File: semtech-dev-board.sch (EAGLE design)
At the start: 58 parts, among them Q1 BSS123, U1 SEMTECH_SX1236, U3 MIC5219 3.3V, X1 BU-SMA-G, X2 BU-SMA-G, X3 BU-SMA-G, X4 BU-SMA-G

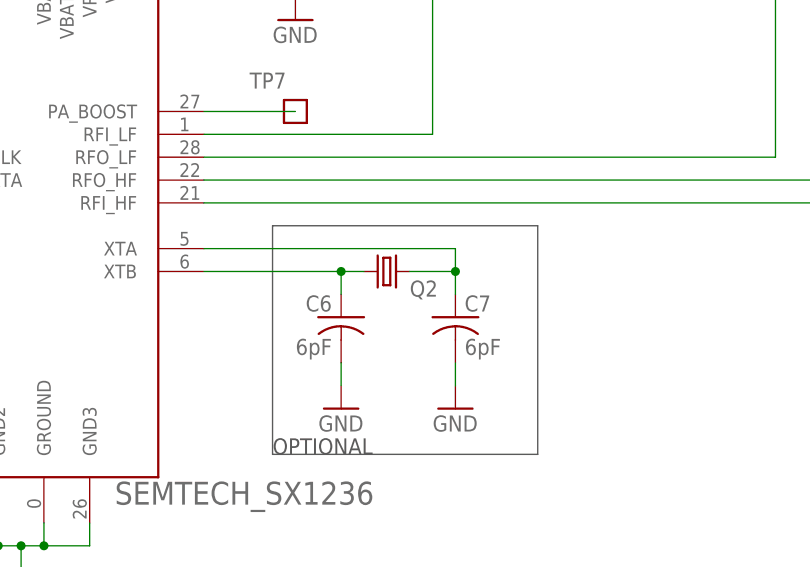
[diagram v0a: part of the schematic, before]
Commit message: minor edits
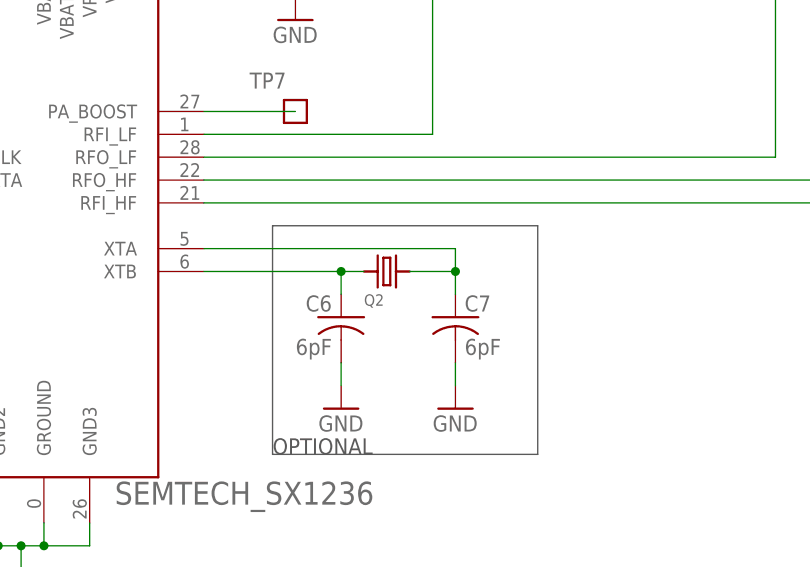
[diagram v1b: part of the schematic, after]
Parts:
- Q2: device crystal:CRYSTALSM49 -> low-gain-radio:CRYSTAL2.5X2.0MM
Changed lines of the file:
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@@
 <grid distance="0.1" unitdist="inch" unit="inch" style="lines" multiple="1" display="no" altdistance="0.01" altunitdist="inch" altunit="inch"/>
 <layers>
-<layer number="1" name="Top" color="4" fill="1" visible="no" active="no"/>
-<layer number="2" name="Route2" color="1" fill="3" visible="no" active="no"/>
-<layer number="3" name="Route3" color="4" fill="3" visible="no" active="no"/>
-<layer number="4" name="Route4" color="1" fill="4" visible="no" active="no"/>
-<layer number="5" name="Route5" color="4" fill="4" visible="no" active="no"/>
-<layer number="6" name="Route6" color="1" fill="8" visible="no" active="no"/>
-<layer number="7" name="Route7" color="4" fill="8" visible="no" active="no"/>
-<layer number="8" name="Route8" color="1" fill="2" visible="no" active="no"/>
-<layer number="9" name="Route9" color="4" fill="2" visible="no" active="no"/>
-<layer number="10" name="Route10" color="1" fill="7" visible="no" active="no"/>
-<layer number="11" name="Route11" color="4" fill="7" visible="no" active="no"/>
-<layer number="12" name="Route12" color="1" fill="5" visible="no" active="no"/>
-<layer number="13" name="Route13" color="4" fill="5" visible="no" active="no"/>
-<layer number="14" name="Route14" color="1" fill="6" visible="no" active="no"/>
-<layer number="15" name="Route15" color="4" fill="6" visible="no" active="no"/>
-<layer number="16" name="Bottom" color="1" fill="1" visible="no" active="no"/>
-<layer number="17" name="Pads" color="2" fill="1" visible="no" active="no"/>
-<layer number="18" name="Vias" color="2" fill="1" visible="no" active="no"/>
-<layer number="19" name="Unrouted" color="6" fill="1" visible="no" active="no"/>
-<layer number="20" name="Dimension" color="15" fill="1" visible="no" active="no"/>
-<layer number="21" name="tPlace" color="7" fill="1" visible="no" active="no"/>
-<layer number="22" name="bPlace" color="7" fill="1" visible="no" active="no"/>
-<layer number="23" name="tOrigins" color="15" fill="1" visible="no" active="no"/>
-<layer number="24" name="bOrigins" color="15" fill="1" visible="no" active="no"/>
-<layer number="25" name="tNames" color="7" fill="1" visible="no" active="no"/>
-<layer number="26" name="bNames" color="7" fill="1" visible="no" active="no"/>
-<layer number="27" name="tValues" color="7" fill="1" visible="no" active="no"/>
-<layer number="28" name="bValues" color="7" fill="1" visible="no" active="no"/>
+<layer number="1" name="Top" color="4" fill="1" visible="yes" active="no"/>
+<layer number="2" name="Route2" color="1" fill="3" visible="yes" active="no"/>
+<layer number="3" name="Route3" color="4" fill="3" visible="yes" active="no"/>
+<layer number="4" name="Route4" color="1" fill="4" visible="yes" active="no"/>
+<layer number="5" name="Route5" color="4" fill="4" visible="yes" active="no"/>
+<layer number="6" name="Route6" color="1" fill="8" visible="yes" active="no"/>
+<layer number="7" name="Route7" color="4" fill="8" visible="yes" active="no"/>
+<layer number="8" name="Route8" color="1" fill="2" visible="yes" active="no"/>
+<layer number="9" name="Route9" color="4" fill="2" visible="yes" active="no"/>
+<layer number="10" name="Route10" color="1" fill="7" visible="yes" active="no"/>
+<layer number="11" name="Route11" color="4" fill="7" visible="yes" active="no"/>
+<layer number="12" name="Route12" color="1" fill="5" visible="yes" active="no"/>
+<layer number="13" name="Route13" color="4" fill="5" visible="yes" active="no"/>
+<layer number="14" name="Route14" color="1" fill="6" visible="yes" active="no"/>
+<layer number="15" name="Route15" color="4" fill="6" visible="yes" active="no"/>
+<layer number="16" name="Bottom" color="1" fill="1" visible="yes" active="no"/>
+<layer number="17" name="Pads" color="2" fill="1" visible="yes" active="no"/>
+<layer number="18" name="Vias" color="2" fill="1" visible="yes" active="no"/>
+<layer number="19" name="Unrouted" color="6" fill="1" visible="yes" active="no"/>
+<layer number="20" name="Dimension" color="15" fill="1" visible="yes" active="no"/>
+<layer number="21" name="tPlace" color="7" fill="1" visible="yes" active="no"/>
+<layer number="22" name="bPlace" color="7" fill="1" visible="yes" active="no"/>
+<layer number="23" name="tOrigins" color="15" fill="1" visible="yes" active="no"/>
+<layer number="24" name="bOrigins" color="15" fill="1" visible="yes" active="no"/>
+<layer number="25" name="tNames" color="7" fill="1" visible="yes" active="no"/>
+<layer number="26" name="bNames" color="7" fill="1" visible="yes" active="no"/>
+<layer number="27" name="tValues" color="7" fill="1" visible="yes" active="no"/>
+<layer number="28" name="bValues" color="7" fill="1" visible="yes" active="no"/>
 <layer number="29" name="tStop" color="7" fill="3" visible="no" active="no"/>
 <layer number="30" name="bStop" color="7" fill="6" visible="no" active="no"/>
@@
 <layer number="35" name="tGlue" color="7" fill="4" visible="no" active="no"/>
 <layer number="36" name="bGlue" color="7" fill="5" visible="no" active="no"/>
-<layer number="37" name="tTest" color="7" fill="1" visible="no" active="no"/>
-<layer number="38" name="bTest" color="7" fill="1" visible="no" active="no"/>
+<layer number="37" name="tTest" color="7" fill="1" visible="yes" active="no"/>
+<layer number="38" name="bTest" color="7" fill="1" visible="yes" active="no"/>
 <layer number="39" name="tKeepout" color="4" fill="11" visible="no" active="no"/>
 <layer number="40" name="bKeepout" color="1" fill="11" visible="no" active="no"/>
@@
 <layer number="44" name="Drills" color="7" fill="1" visible="no" active="no"/>
 <layer number="45" name="Holes" color="7" fill="1" visible="no" active="no"/>
-<layer number="46" name="Milling" color="3" fill="1" visible="no" active="no"/>
-<layer number="47" name="Measures" color="7" fill="1" visible="no" active="no"/>
-<layer number="48" name="Document" color="7" fill="1" visible="no" active="no"/>
-<layer number="49" name="Reference" color="7" fill="1" visible="no" active="no"/>
-<layer number="50" name="dxf" color="7" fill="1" visible="no" active="no"/>
-<layer number="51" name="tDocu" color="7" fill="1" visible="no" active="no"/>
-<layer number="52" name="bDocu" color="7" fill="1" visible="no" active="no"/>
-<layer number="53" name="tGND_GNDA" color="7" fill="1" visible="no" active="no"/>
-<layer number="54" name="bGND_GNDA" color="7" fill="1" visible="no" active="no"/>
-<layer number="56" name="wert" color="7" fill="1" visible="no" active="no"/>
-<layer number="57" name="tCAD" color="7" fill="1" visible="no" active="no"/>
-<layer number="58" name="b3D" color="7" fill="1" visible="no" active="no"/>
-<layer number="59" name="Invisible" color="7" fill="1" visible="no" active="no"/>
-<layer number="60" name="bCarbon" color="7" fill="1" visible="no" active="no"/>
-<layer number="61" name="stand" color="7" fill="1" visible="no" active="no"/>
+<layer number="46" name="Milling" color="3" fill="1" visible="yes" active="no"/>
+<layer number="47" name="Measures" color="7" fill="1" visible="yes" active="no"/>
+<layer number="48" name="Document" color="7" fill="1" visible="yes" active="no"/>
+<layer number="49" name="Reference" color="7" fill="1" visible="yes" active="no"/>
+<layer number="50" name="dxf" color="7" fill="1" visible="yes" active="no"/>
+<layer number="51" name="tDocu" color="7" fill="1" visible="yes" active="no"/>
+<layer number="52" name="bDocu" color="7" fill="1" visible="yes" active="no"/>
+<layer number="53" name="tGND_GNDA" color="7" fill="1" visible="yes" active="no"/>
+<layer number="54" name="bGND_GNDA" color="7" fill="1" visible="yes" active="no"/>
+<layer number="56" name="wert" color="7" fill="1" visible="yes" active="no"/>
+<layer number="57" name="tCAD" color="7" fill="1" visible="yes" active="no"/>
+<layer number="58" name="b3D" color="7" fill="1" visible="yes" active="no"/>
+<layer number="59" name="Invisible" color="7" fill="1" visible="yes" active="no"/>
+<layer number="60" name="bCarbon" color="7" fill="1" visible="yes" active="no"/>
+<layer number="61" name="stand" color="7" fill="1" visible="yes" active="no"/>
 <layer number="90" name="Modules" color="5" fill="1" visible="yes" active="yes"/>
 <layer number="91" name="Nets" color="2" fill="1" visible="yes" active="yes"/>
@@
 <part name="X2" library="con-coax" deviceset="BU-SMA-G" device=""/>
 <part name="X3" library="con-coax" deviceset="BU-SMA-G" device=""/>
-<part name="Q2" library="crystal" deviceset="CRYSTAL" device="SM49"/>
+<part name="Q2" library="low-gain-radio" deviceset="CRYSTAL" device="2.5X2.0MM"/>
 <part name="S1" library="switch" deviceset="RDT1034" device=""/>
 <part name="GND2" library="supply1" deviceset="GND" device=""/>
